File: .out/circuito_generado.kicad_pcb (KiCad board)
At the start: 2 copper layers, 100 x 70 mm, 4 parts

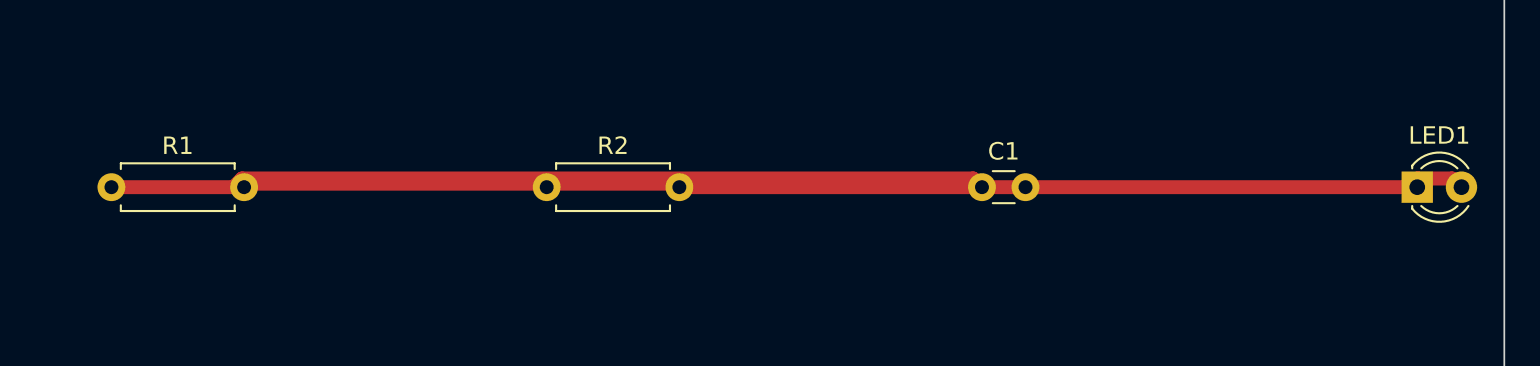
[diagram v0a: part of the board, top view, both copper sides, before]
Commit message: Version v1.0.4
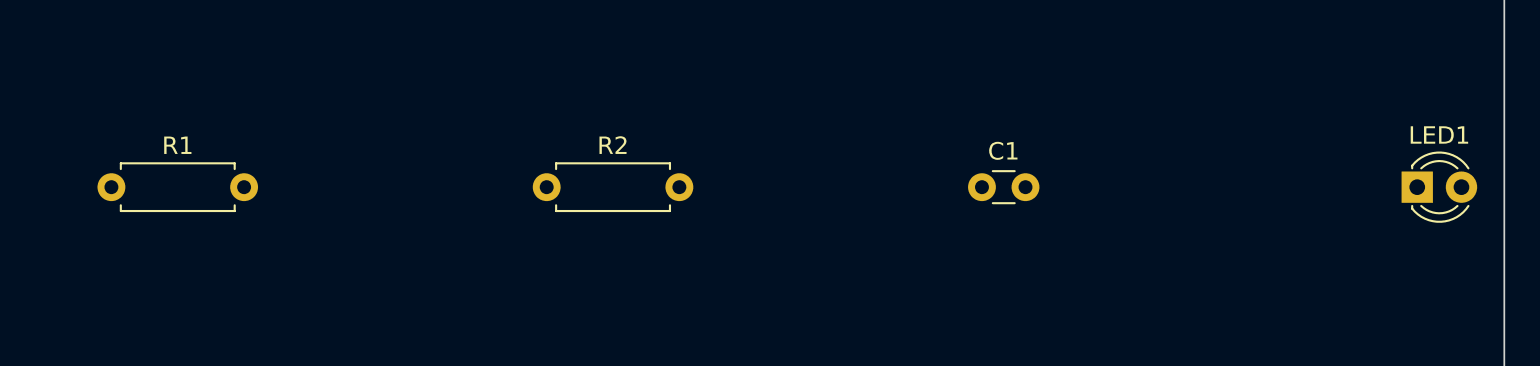
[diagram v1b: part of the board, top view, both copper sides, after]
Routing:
- net NET1: track 67.5 -> 0.00 mm
- net VCC: track 50.4 -> 0.00 mm
- net GND: track 45.4 -> 0.00 mm
